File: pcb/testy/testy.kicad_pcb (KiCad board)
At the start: 2 copper layers, 144.9 x 102 mm, 83 parts, among them J1 Conn_01x02, J2 Conn_01x02, SW0:0 SW_Push, SW0:1 SW_Push, SW0:2 SW_Push, SW0:3 SW_Push, SW0:4 SW_Push, SW0:5 SW_Push, SW1:0 SW_Push, SW1:1 SW_Push, SW1:2 SW_Push, SW1:3 SW_Push, SW1:4 SW_Push, SW1:5 SW_Push, SW2:0 SW_Push, SW2:1 SW_Push, SW2:2 SW_Push, SW2:3 SW_Push, SW2:4 SW_Push, SW2:5 SW_Push, SW3:0 SW_Push, SW3:1 SW_Push, SW3:2 SW_Push, SW3:3 SW_Push, SW3:4 SW_Push, SW3:5 SW_Push, SW3:6 SW_Push, SW4:0 SW_Push, SW4:1 SW_Push, SW4:2 SW_Push, SW4:3 SW_Push, SW4:4 SW_Push, SW4:5 SW_Push, SW4:6 SW_Push, U1 ProMicro

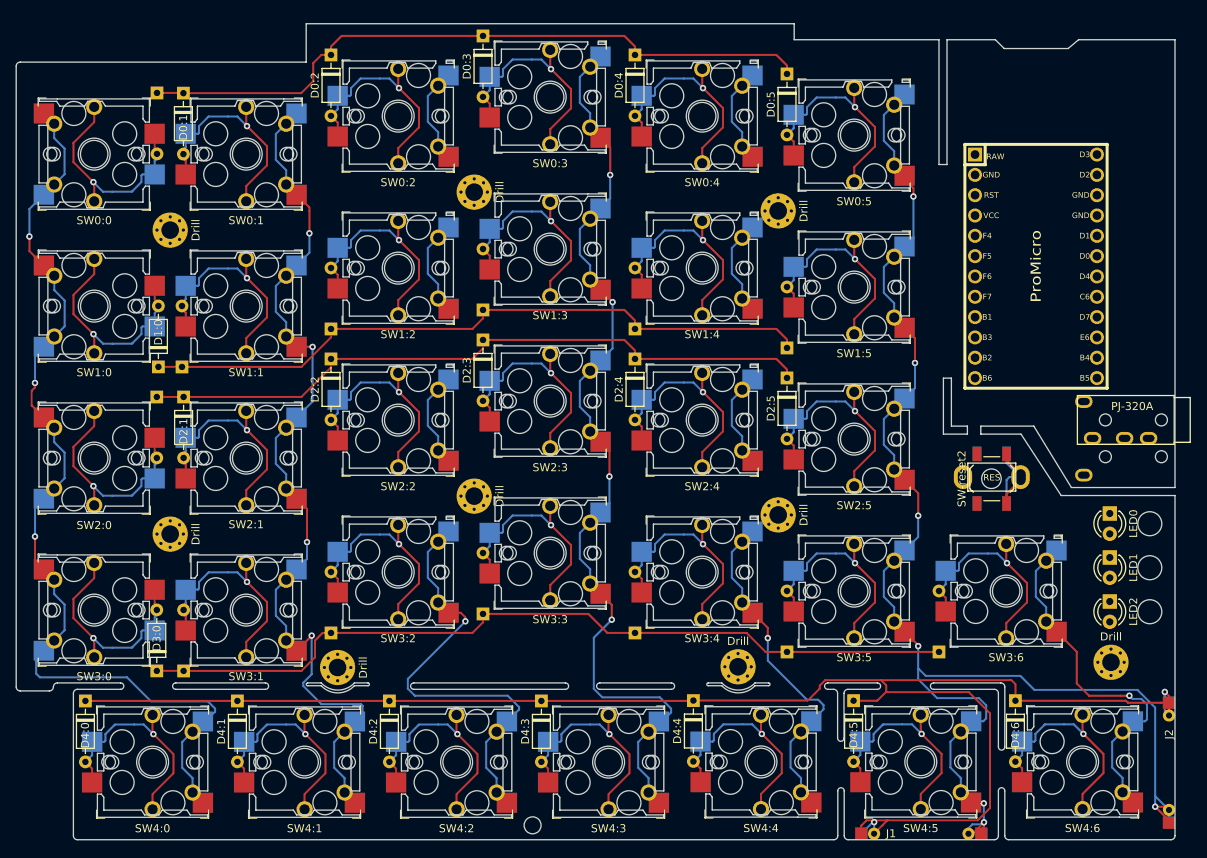
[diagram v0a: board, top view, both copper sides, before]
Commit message: feat: move to new 5 col version
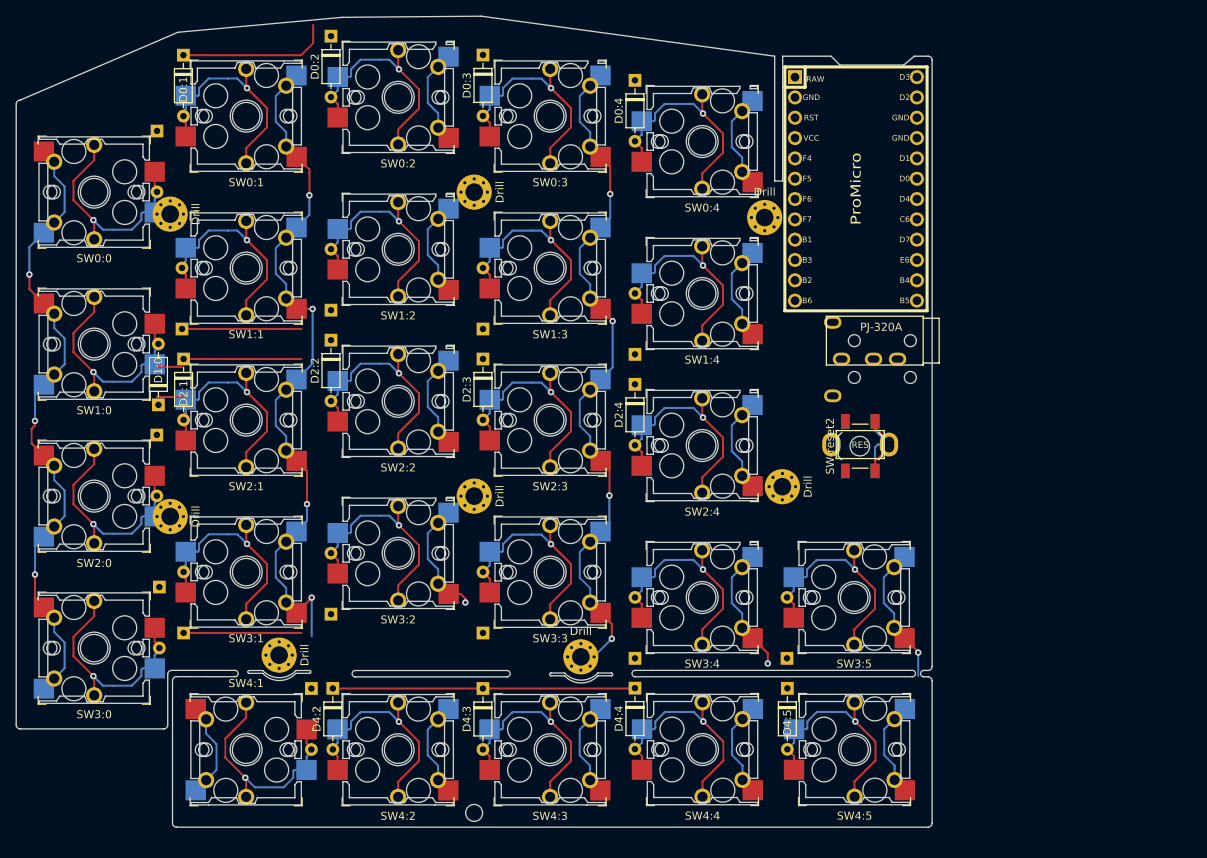
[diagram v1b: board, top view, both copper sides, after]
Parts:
- removed D0:5, D1:5, D2:5, D3:6, D4:0, D4:6: 1N4148, Diode_THT:D_DO-35_SOD27_P7.62mm_Horizontal
- removed the Drill at (167.7, 68.4)
- removed J1, J2: Conn_01x02, footprints:edge-connector
- removed LED0: LED, footprints:LED_D3.0mm
- removed LED1, LED2: LED, LED_THT:LED_D3.0mm
- removed SW0:5, SW1:5, SW2:5, SW3:6, SW4:0, SW4:6: SW_Push, footprints:kailh-socket-and-choc-solder-reversible
- D3:0, D4:1: moved to B.Cu
- moved Drill 70.5 mm to (166.0, 69.2)
- moved TRRS1 32.9 mm to (185.8, 86.9)
- moved U1 24.5 mm to (177.4, 64.1)
- moved Drill 19.7 mm to (143.0, 124.1)
- moved SW-reset1 16.9 mm to (177.9, 99.4)
- moved SW-reset2 16.9 mm to (177.9, 97.8)
- moved SW-reset3 16.9 mm to (177.9, 97.8)
- moved D3:0 10.5 mm to (90.3, 115.4), turned to 270 degrees
- moved D4:1 9.38 mm to (109.3, 128.1)
- moved D4:5 8.42 mm to (168.8, 128.1)
- moved SW4:5 8.42 mm to (177.2, 135.7)
- moved D4:3 7.47 mm to (130.8, 128.1)
- moved SW4:1 7.47 mm to (101.2, 135.8), turned to 180 degrees
- moved SW4:2 7.47 mm to (120.2, 135.8)
- moved SW4:3 7.47 mm to (139.2, 135.8)
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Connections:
- net Net-(U1-Pad13) renamed LED
- net Net-(U1-Pad17) renamed SDA
- U1 pad 12: LED2 -> Net-(U1-Pad12)
- U1 pad 18: LED0 -> SCL
- U1 pad 24: LED1 -> Net-(U1-Pad24)
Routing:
- net Row4: track 203.5 -> 38.0 mm, vias 2 -> 0
- net Col5: track 177.1 -> 30.0 mm, vias 7 -> 1
- net Row3: track 104.5 -> 14.7 mm
- net Row2: track 86.2 -> 18.1 mm
- net Row1: track 86.0 -> 17.9 mm
- net Row0: track 86.9 -> 19.1 mm
- net Col6: track 45.8 -> 0.00 mm, vias 1 -> 0
- net Col0: track 121.8 -> 79.6 mm
- net Net-(D2:5-Pad2): track 29.1 -> 0.00 mm, vias 1 -> 0
- net Net-(D0:5-Pad2): track 29.1 -> 0.00 mm, vias 1 -> 0
- net Net-(D4:6-Pad2): track 29.1 -> 0.00 mm, vias 1 -> 0
- net Net-(D4:0-Pad2): track 29.1 -> 0.00 mm, vias 1 -> 0
- net Net-(D3:6-Pad2): track 29.1 -> 0.00 mm, vias 1 -> 0
- net Net-(D1:5-Pad2): track 29.1 -> 0.00 mm, vias 1 -> 0
- net Col2: track 93.2 -> 64.5 mm
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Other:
- board size 144.9 x 102 mm -> 114.5 x 101.4 mm
- board text added: "TODO add WSxxxx LED here?"
- board text added: "TODO add cuts around promicro, etc"
- board text added: "TODO align SW4:4 properly"
- board text removed: "<-- add mount for USB-C breakout board Only need mechanical mounting as electrically it'll be a flying lead"
- board text removed: "<-- add snapoff piece that can be soldered in as a thumb rest when SW4:5 is moved"
- board text removed: "<-- are edge fingers ok, or should we do through holes an mount the extra piece slight higher? Wire pads up in schematic"
- board text removed: "<-- look at moving ProMicro lower so USB-C breakout and protrude and protect the flying lead for the PM, but still be inside the rectangle footprint"
- board text removed: "TODO add resistors for LEDs"
